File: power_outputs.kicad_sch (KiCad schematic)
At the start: 10 parts, among them Q1 BSS138, Q3 MMBT3904, Q4 MMBT3906

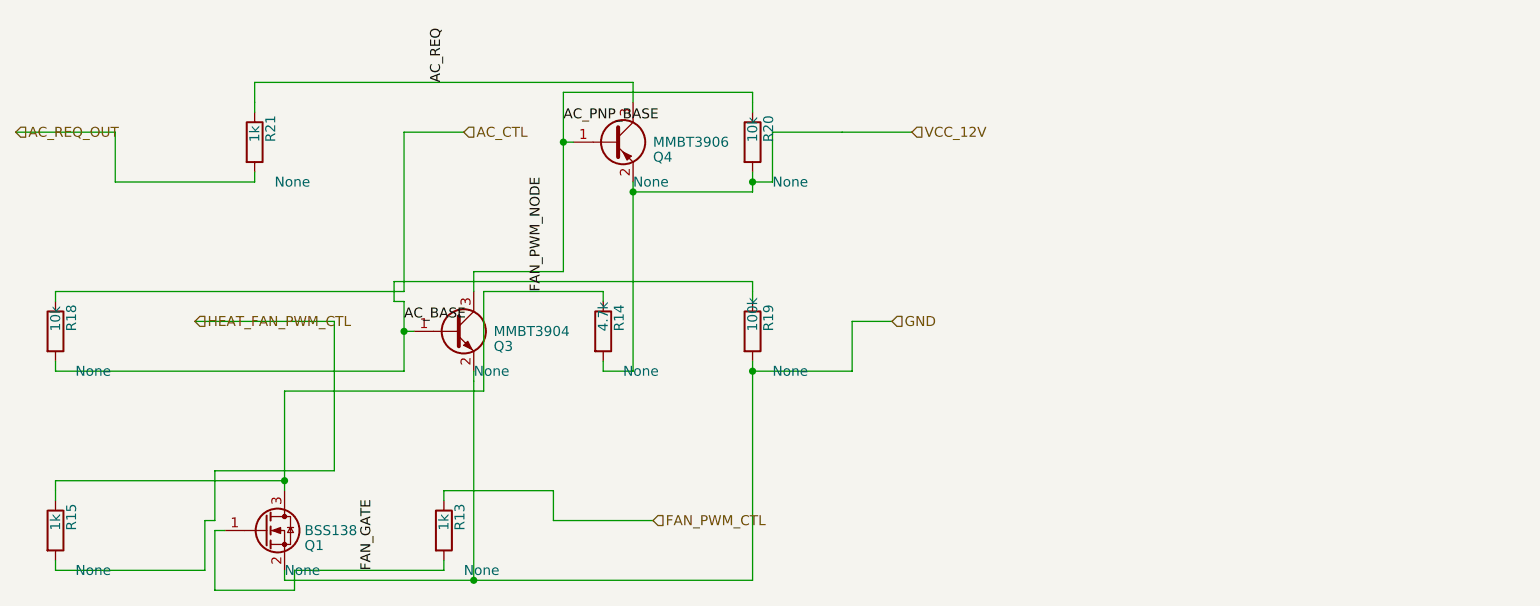
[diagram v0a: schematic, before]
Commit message: tests_fix
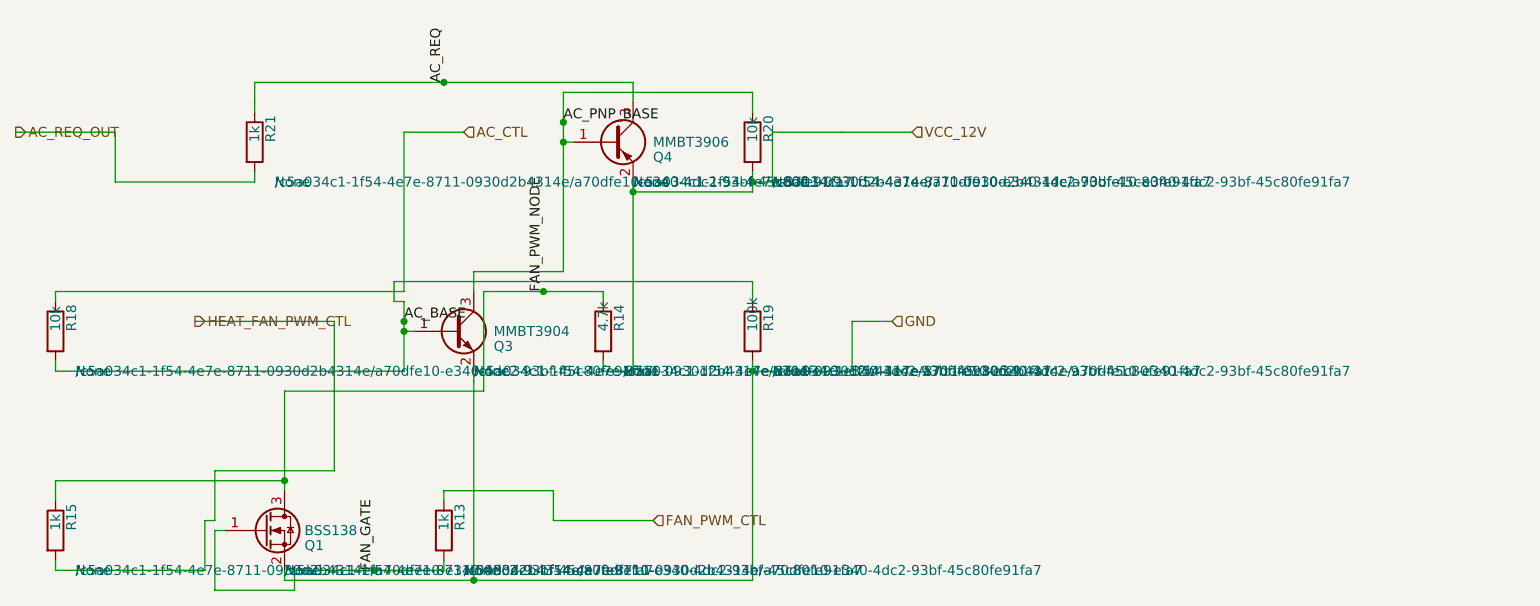
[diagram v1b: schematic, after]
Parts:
- Q1, Q3, Q4, R13, R14, R15, R18, R19, R20, R21: hierarchy_path (none) -> /c5a034c1-1f54-4e7e-8711-0930d2b4314e/a70dfe10-e340-4dc2-93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
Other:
- title: (none) -> climate_control_niva_travel
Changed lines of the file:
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@@
 	(generator_version "9.0")
 	(paper "A4")
+	(title_block
+		(title "climate_control_niva_travel")
+	)
 	(symbol
 		(lib_id "Transistor_FET:BSS138")
@@
 			)
 		)
+		(property "hierarchy_path" "/c5a034c1-1f54-4e7e-8711-0930d2b4314e/a70dfe10-e340-4dc2-93bf-45c80fe91fa7"
+			(at 38.1 63.4999 0)
+			(effects
+				(font
+					(size 1.27 1.27)
+				)
+				(justify left)
+			)
+		)
 		(pin "1"
 		)
@@
 		)
 		(instances
-			(project "Untitled"
-				(path "/90d6963e-6ac5-4f32-9aa0-e0ee6a940a9b"
+			(project "climate_control_niva_travel"
+				(path "/c5a034c1-1f54-4e7e-8711-0930d2b4314e/a70dfe10-e340-4dc2-93bf-45c80fe91fa7"
 					(reference "Q1")
 					(unit 1)
@@
 			)
 		)
+		(property "hierarchy_path" "/c5a034c1-1f54-4e7e-8711-0930d2b4314e/a70dfe10-e340-4dc2-93bf-45c80fe91fa7"
+			(at 62.23 38.0999 0)
+			(effects
+				(font
+					(size 1.27 1.27)
+				)
+				(justify left)
+			)
+		)
 		(pin "1"
 		)
@@
 		)
 		(instances
-			(project "Untitled"
-				(path "/90d6963e-6ac5-4f32-9aa0-e0ee6a940a9b"
+			(project "climate_control_niva_travel"
+				(path "/c5a034c1-1f54-4e7e-8711-0930d2b4314e/a70dfe10-e340-4dc2-93bf-45c80fe91fa7"
 					(reference "Q3")
 					(unit 1)
@@
 			)
 		)
+		(property "hierarchy_path" "/c5a034c1-1f54-4e7e-8711-0930d2b4314e/a70dfe10-e340-4dc2-93bf-45c80fe91fa7"
+			(at 82.55 13.9699 0)
+			(effects
+				(font
+					(size 1.27 1.27)
+				)
+				(justify left)
+			)
+		)
 		(pin "1"
 		)
@@
 		)
 		(instances
-			(project "Untitled"
-				(path "/90d6963e-6ac5-4f32-9aa0-e0ee6a940a9b"
+			(project "climate_control_niva_travel"
+				(path "/c5a034c1-1f54-4e7e-8711-0930d2b4314e/a70dfe10-e340-4dc2-93bf-45c80fe91fa7"
 					(reference "Q4")
 					(unit 1)
@@
 			)
 		)
+		(property "hierarchy_path" "/c5a034c1-1f54-4e7e-8711-0930d2b4314e/a70dfe10-e340-4dc2-93bf-45c80fe91fa7"
+			(at 60.96 63.4999 0)
+			(effects
+				(font
+					(size 1.27 1.27)
+				)
+				(justify left)
+			)
+		)
 		(pin "1"
 		)
@@
 		)
 		(instances
-			(project "Untitled"
-				(path "/90d6963e-6ac5-4f32-9aa0-e0ee6a940a9b"
+			(project "climate_control_niva_travel"
+				(path "/c5a034c1-1f54-4e7e-8711-0930d2b4314e/a70dfe10-e340-4dc2-93bf-45c80fe91fa7"
 					(reference "R13")
 					(unit 1)
@@
 			)
 		)
+		(property "hierarchy_path" "/c5a034c1-1f54-4e7e-8711-0930d2b4314e/a70dfe10-e340-4dc2-93bf-45c80fe91fa7"
+			(at 81.28 38.0999 0)
+			(effects
+				(font
+					(size 1.27 1.27)
+				)
+				(justify left)
+			)
+		)
 		(pin "1"
 		)
@@
 		)
 		(instances
-			(project "Untitled"
-				(path "/90d6963e-6ac5-4f32-9aa0-e0ee6a940a9b"
+			(project "climate_control_niva_travel"
+				(path "/c5a034c1-1f54-4e7e-8711-0930d2b4314e/a70dfe10-e340-4dc2-93bf-45c80fe91fa7"
 					(reference "R14")
 					(unit 1)
@@
 			)
 		)
+		(property "hierarchy_path" "/c5a034c1-1f54-4e7e-8711-0930d2b4314e/a70dfe10-e340-4dc2-93bf-45c80fe91fa7"
+			(at 11.43 63.4999 0)
+			(effects
+				(font
+					(size 1.27 1.27)
+				)
+				(justify left)
+			)
+		)
 		(pin "1"
 		)
@@
 		)
 		(instances
-			(project "Untitled"
-				(path "/90d6963e-6ac5-4f32-9aa0-e0ee6a940a9b"
+			(project "climate_control_niva_travel"
+				(path "/c5a034c1-1f54-4e7e-8711-0930d2b4314e/a70dfe10-e340-4dc2-93bf-45c80fe91fa7"
 					(reference "R15")
 					(unit 1)
@@
 			)
 		)
+		(property "hierarchy_path" "/c5a034c1-1f54-4e7e-8711-0930d2b4314e/a70dfe10-e340-4dc2-93bf-45c80fe91fa7"
+			(at 11.43 38.0999 0)
+			(effects
+				(font
+					(size 1.27 1.27)
+				)
+				(justify left)
+			)
+		)
 		(pin "1"
 		)
@@
 		)
 		(instances
-			(project "Untitled"
-				(path "/90d6963e-6ac5-4f32-9aa0-e0ee6a940a9b"
+			(project "climate_control_niva_travel"
+				(path "/c5a034c1-1f54-4e7e-8711-0930d2b4314e/a70dfe10-e340-4dc2-93bf-45c80fe91fa7"
 					(reference "R18")
 					(unit 1)
@@
 			)
 		)
+		(property "hierarchy_path" "/c5a034c1-1f54-4e7e-8711-0930d2b4314e/a70dfe10-e340-4dc2-93bf-45c80fe91fa7"
+			(at 100.33 38.0999 0)
+			(effects
+				(font
+					(size 1.27 1.27)
+				)
+				(justify left)
+			)
+		)
 		(pin "1"
 		)
@@
 		)
 		(instances
-			(project "Untitled"
-				(path "/90d6963e-6ac5-4f32-9aa0-e0ee6a940a9b"
+			(project "climate_control_niva_travel"
+				(path "/c5a034c1-1f54-4e7e-8711-0930d2b4314e/a70dfe10-e340-4dc2-93bf-45c80fe91fa7"
 					(reference "R19")
 					(unit 1)
@@
 			)
 		)
+		(property "hierarchy_path" "/c5a034c1-1f54-4e7e-8711-0930d2b4314e/a70dfe10-e340-4dc2-93bf-45c80fe91fa7"
+			(at 100.33 13.9699 0)
+			(effects
+				(font
+					(size 1.27 1.27)
+				)
+				(justify left)
+			)
+		)
 		(pin "1"
 		)
@@
 		)
 		(instances
-			(project "Untitled"
-				(path "/90d6963e-6ac5-4f32-9aa0-e0ee6a940a9b"
+			(project "climate_control_niva_travel"
+				(path "/c5a034c1-1f54-4e7e-8711-0930d2b4314e/a70dfe10-e340-4dc2-93bf-45c80fe91fa7"
 					(reference "R20")
 					(unit 1)
@@
 			)
 		)
+		(property "hierarchy_path" "/c5a034c1-1f54-4e7e-8711-0930d2b4314e/a70dfe10-e340-4dc2-93bf-45c80fe91fa7"
+			(at 36.83 13.9699 0)
+			(effects
+				(font
+					(size 1.27 1.27)
+				)
+				(justify left)
+			)
+		)
 		(pin "1"
 		)
@@
 		)
 		(instances
-			(project "Untitled"
-				(path "/90d6963e-6ac5-4f32-9aa0-e0ee6a940a9b"
+			(project "climate_control_niva_travel"
+				(path "/c5a034c1-1f54-4e7e-8711-0930d2b4314e/a70dfe10-e340-4dc2-93bf-45c80fe91fa7"
 					(reference "R21")
 					(unit 1)
@@
 	(junction
 		(at 73.66 8.89)
+		(diameter 0)
+		(color 0 0 0 0)
+	)
+	(junction
+		(at 49.53 63.5)
+		(diameter 0)
+		(color 0 0 0 0)
+	)
+	(junction
+		(at 71.12 27.94)
+		(diameter 0)
+		(color 0 0 0 0)
+	)
+	(junction
+		(at 53.34 31.75)
+		(diameter 0)
+		(color 0 0 0 0)
+	)
+	(junction
+		(at 73.66 6.35)
+		(diameter 0)
+		(color 0 0 0 0)
+	)
+	(junction
+		(at 58.42 1.27)
 		(diameter 0)
 		(color 0 0 0 0)
@@
 	)
 	(hierarchical_label "AC_REQ_OUT"
-		(shape input)
+		(shape output)
 		(at 3.81 7.62 0)
 		(effects
@@
 	)
 	(hierarchical_label "HEAT_FAN_PWM_CTL"
-		(shape input)
+		(shape output)
 		(at 26.67 31.75 0)
 		(effects

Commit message: refactoring
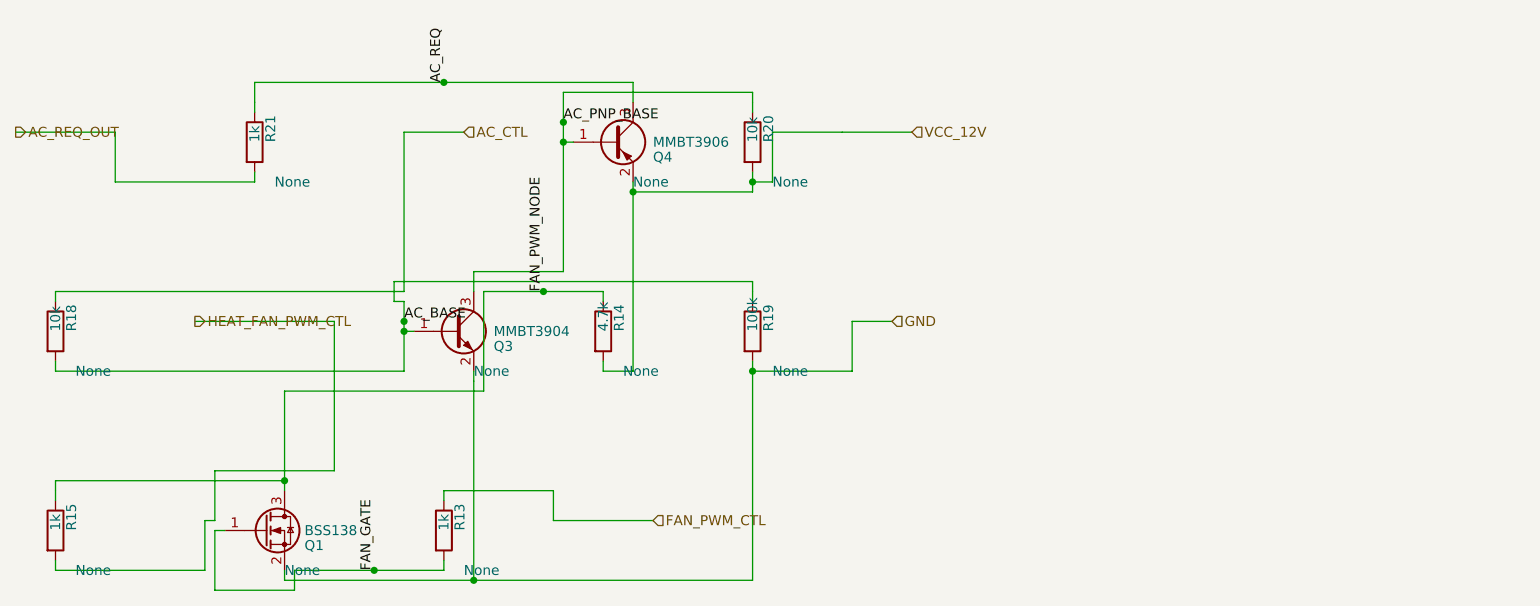
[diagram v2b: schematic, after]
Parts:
- Q1, Q3, Q4, R13, R14, R15, R18, R19, R20, R21: hierarchy_path /c5a034c1-1f54-4e7e-8711-0930d2b4314e/a70dfe10-e340-4dc2-93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 -> (none)
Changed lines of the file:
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@@
-			)
-		)
-		(property "hierarchy_path" "/c5a034c1-1f54-4e7e-8711-0930d2b4314e/a70dfe10-e340-4dc2-93bf-45c80fe91fa7"
-			(at 38.1 63.4999 0)
-			(effects
-				(font
-					(size 1.27 1.27)
-				)
-				(justify left)
 			)
 		)
@@
 		(instances
 			(project "climate_control_niva_travel"
-				(path "/c5a034c1-1f54-4e7e-8711-0930d2b4314e/a70dfe10-e340-4dc2-93bf-45c80fe91fa7"
-					(reference "Q1")
+				(path "/165a98f1-2dde-4141-9fdc-c935d39c8cff/176bfc83-1f39-4dbb-bd36-1c3de8b994cb/"
+					(reference "Q0701")
 					(unit 1)
 				)
@@
 			)
 		)
-		(property "hierarchy_path" "/c5a034c1-1f54-4e7e-8711-0930d2b4314e/a70dfe10-e340-4dc2-93bf-45c80fe91fa7"
-			(at 62.23 38.0999 0)
-			(effects
-				(font
-					(size 1.27 1.27)
-				)
-				(justify left)
-			)
-		)
 		(pin "1"
 		)
@@
 		(instances
 			(project "climate_control_niva_travel"
-				(path "/c5a034c1-1f54-4e7e-8711-0930d2b4314e/a70dfe10-e340-4dc2-93bf-45c80fe91fa7"
-					(reference "Q3")
+				(path "/165a98f1-2dde-4141-9fdc-c935d39c8cff/176bfc83-1f39-4dbb-bd36-1c3de8b994cb/"
+					(reference "Q0703")
 					(unit 1)
 				)
@@
 			)
 		)
-		(property "hierarchy_path" "/c5a034c1-1f54-4e7e-8711-0930d2b4314e/a70dfe10-e340-4dc2-93bf-45c80fe91fa7"
-			(at 82.55 13.9699 0)
-			(effects
-				(font
-					(size 1.27 1.27)
-				)
-				(justify left)
-			)
-		)
 		(pin "1"
 		)
@@
 		(instances
 			(project "climate_control_niva_travel"
-				(path "/c5a034c1-1f54-4e7e-8711-0930d2b4314e/a70dfe10-e340-4dc2-93bf-45c80fe91fa7"
-					(reference "Q4")
+				(path "/165a98f1-2dde-4141-9fdc-c935d39c8cff/176bfc83-1f39-4dbb-bd36-1c3de8b994cb/"
+					(reference "Q0704")
 					(unit 1)
 				)
@@
 			)
 		)
-		(property "hierarchy_path" "/c5a034c1-1f54-4e7e-8711-0930d2b4314e/a70dfe10-e340-4dc2-93bf-45c80fe91fa7"
-			(at 60.96 63.4999 0)
-			(effects
-				(font
-					(size 1.27 1.27)
-				)
-				(justify left)
-			)
-		)
-		(pin "1"
-		)
-		(pin "2"
-		)
-		(instances
-			(project "climate_control_niva_travel"
-				(path "/c5a034c1-1f54-4e7e-8711-0930d2b4314e/a70dfe10-e340-4dc2-93bf-45c80fe91fa7"
-					(reference "R13")
+		(pin "1"
+		)
+		(pin "2"
+		)
+		(instances
+			(project "climate_control_niva_travel"
+				(path "/165a98f1-2dde-4141-9fdc-c935d39c8cff/176bfc83-1f39-4dbb-bd36-1c3de8b994cb/"
+					(reference "R0713")
 					(unit 1)
 				)
@@
 			)
 		)
-		(property "hierarchy_path" "/c5a034c1-1f54-4e7e-8711-0930d2b4314e/a70dfe10-e340-4dc2-93bf-45c80fe91fa7"
-			(at 81.28 38.0999 0)
-			(effects
-				(font
-					(size 1.27 1.27)
-				)
-				(justify left)
-			)
-		)
-		(pin "1"
-		)
-		(pin "2"
-		)
-		(instances
-			(project "climate_control_niva_travel"
-				(path "/c5a034c1-1f54-4e7e-8711-0930d2b4314e/a70dfe10-e340-4dc2-93bf-45c80fe91fa7"
-					(reference "R14")
+		(pin "1"
+		)
+		(pin "2"
+		)
+		(instances
+			(project "climate_control_niva_travel"
+				(path "/165a98f1-2dde-4141-9fdc-c935d39c8cff/176bfc83-1f39-4dbb-bd36-1c3de8b994cb/"
+					(reference "R0714")
 					(unit 1)
 				)
@@
 			)
 		)
-		(property "hierarchy_path" "/c5a034c1-1f54-4e7e-8711-0930d2b4314e/a70dfe10-e340-4dc2-93bf-45c80fe91fa7"
-			(at 11.43 63.4999 0)
-			(effects
-				(font
-					(size 1.27 1.27)
-				)
-				(justify left)
-			)
-		)
-		(pin "1"
-		)
-		(pin "2"
-		)
-		(instances
-			(project "climate_control_niva_travel"
-				(path "/c5a034c1-1f54-4e7e-8711-0930d2b4314e/a70dfe10-e340-4dc2-93bf-45c80fe91fa7"
-					(reference "R15")
+		(pin "1"
+		)
+		(pin "2"
+		)
+		(instances
+			(project "climate_control_niva_travel"
+				(path "/165a98f1-2dde-4141-9fdc-c935d39c8cff/176bfc83-1f39-4dbb-bd36-1c3de8b994cb/"
+					(reference "R0715")
 					(unit 1)
 				)
@@
 			)
 		)
-		(property "hierarchy_path" "/c5a034c1-1f54-4e7e-8711-0930d2b4314e/a70dfe10-e340-4dc2-93bf-45c80fe91fa7"
-			(at 11.43 38.0999 0)
-			(effects
-				(font
-					(size 1.27 1.27)
-				)
-				(justify left)
-			)
-		)
-		(pin "1"
-		)
-		(pin "2"
-		)
-		(instances
-			(project "climate_control_niva_travel"
-				(path "/c5a034c1-1f54-4e7e-8711-0930d2b4314e/a70dfe10-e340-4dc2-93bf-45c80fe91fa7"
-					(reference "R18")
+		(pin "1"
+		)
+		(pin "2"
+		)
+		(instances
+			(project "climate_control_niva_travel"
+				(path "/165a98f1-2dde-4141-9fdc-c935d39c8cff/176bfc83-1f39-4dbb-bd36-1c3de8b994cb/"
+					(reference "R0718")
 					(unit 1)
 				)
@@
 			)
 		)
-		(property "hierarchy_path" "/c5a034c1-1f54-4e7e-8711-0930d2b4314e/a70dfe10-e340-4dc2-93bf-45c80fe91fa7"
-			(at 100.33 38.0999 0)
-			(effects
-				(font
-					(size 1.27 1.27)
-				)
-				(justify left)
-			)
-		)
-		(pin "1"
-		)
-		(pin "2"
-		)
-		(instances
-			(project "climate_control_niva_travel"
-				(path "/c5a034c1-1f54-4e7e-8711-0930d2b4314e/a70dfe10-e340-4dc2-93bf-45c80fe91fa7"
-					(reference "R19")
+		(pin "1"
+		)
+		(pin "2"
+		)
+		(instances
+			(project "climate_control_niva_travel"
+				(path "/165a98f1-2dde-4141-9fdc-c935d39c8cff/176bfc83-1f39-4dbb-bd36-1c3de8b994cb/"
+					(reference "R0719")
 					(unit 1)
 				)
@@
 			)
 		)
-		(property "hierarchy_path" "/c5a034c1-1f54-4e7e-8711-0930d2b4314e/a70dfe10-e340-4dc2-93bf-45c80fe91fa7"
-			(at 100.33 13.9699 0)
-			(effects
-				(font
-					(size 1.27 1.27)
-				)
-				(justify left)
-			)
-		)
-		(pin "1"
-		)
-		(pin "2"
-		)
-		(instances
-			(project "climate_control_niva_travel"
-				(path "/c5a034c1-1f54-4e7e-8711-0930d2b4314e/a70dfe10-e340-4dc2-93bf-45c80fe91fa7"
-					(reference "R20")
+		(pin "1"
+		)
+		(pin "2"
+		)
+		(instances
+			(project "climate_control_niva_travel"
+				(path "/165a98f1-2dde-4141-9fdc-c935d39c8cff/176bfc83-1f39-4dbb-bd36-1c3de8b994cb/"
+					(reference "R0720")
 					(unit 1)
 				)
@@
 			)
 		)
-		(property "hierarchy_path" "/c5a034c1-1f54-4e7e-8711-0930d2b4314e/a70dfe10-e340-4dc2-93bf-45c80fe91fa7"
-			(at 36.83 13.9699 0)
-			(effects
-				(font
-					(size 1.27 1.27)
-				)
-				(justify left)
-			)
-		)
-		(pin "1"
-		)
-		(pin "2"
-		)
-		(instances
-			(project "climate_control_niva_travel"
-				(path "/c5a034c1-1f54-4e7e-8711-0930d2b4314e/a70dfe10-e340-4dc2-93bf-45c80fe91fa7"
-					(reference "R21")
-					(unit 1)
-				)
+		(pin "1"
+		)
+		(pin "2"
+		)
+		(instances
+			(project "climate_control_niva_travel"
+				(path "/165a98f1-2dde-4141-9fdc-c935d39c8cff/176bfc83-1f39-4dbb-bd36-1c3de8b994cb/"
+					(reference "R0721")
+					(unit 1)
+				)

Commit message: refactoring
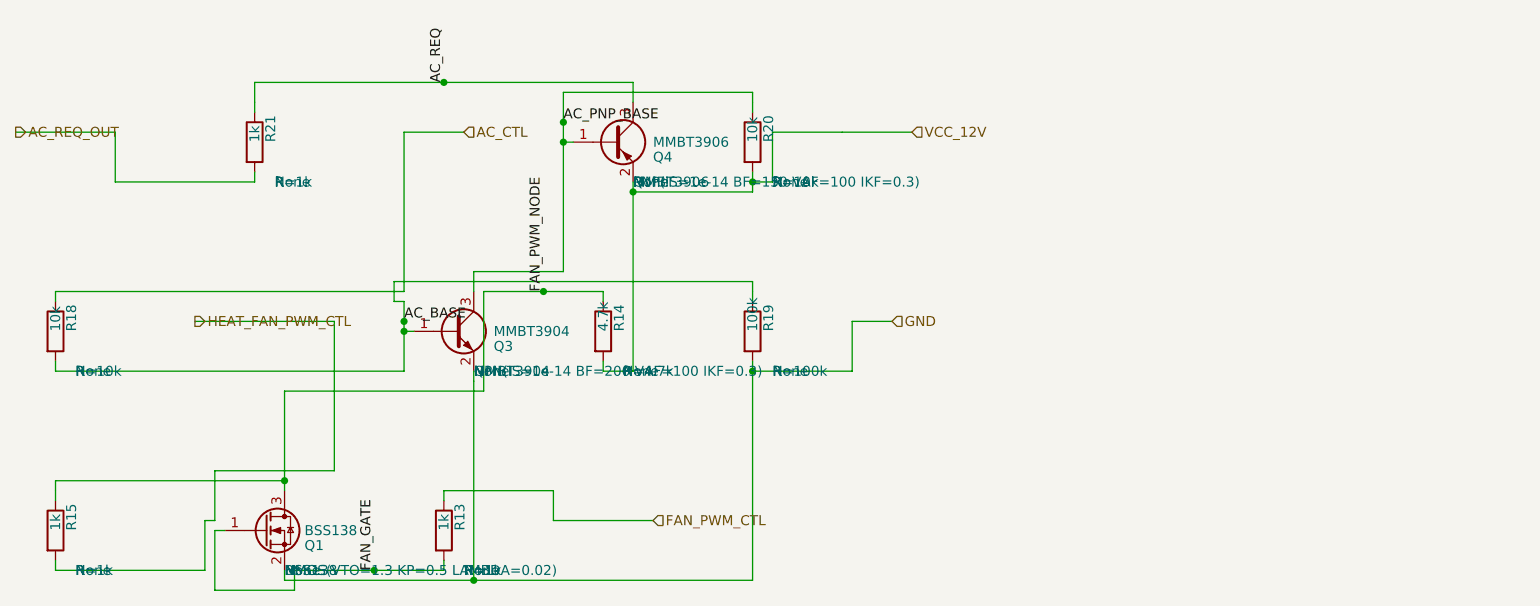
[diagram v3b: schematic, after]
